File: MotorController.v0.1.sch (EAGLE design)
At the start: 47 parts, among them IC1 MC33035, IC2 MC33039

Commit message: Image + version.
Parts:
- removed R3B: 1M, resistor:R-EU_0204/2V
- added C2: 0.01uF, rcl:C-EU025-025X050
- added C6: 47uF, rcl:C-EU025-025X050
- added D5: 1N4148, diode:1N4148DO35-7
- added JP2: (no value), jumper:JP1E
- added LED1: (no value), led:LEDLD260
- added R10, R11: 2.2k, resistor:R-EU_0204/2V
- added R19: 4.7k, resistor:R-EU_0204/2V
- added SL2: (no value), con-amp-quick:M02
- R2: value 1M -> 5.1k
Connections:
- removed net FAULT: IC1.14
- new net FAULT_N: D5.C, IC1.14, LED1.C
- new net FOUT_: JP2.1, R3.1, TP1.TP
- new net FWD/REV: IC1.3, S1.S
- new net N$1: R19.1, S2.S
- new net N$11: C6.1, INC.3, R10.1, S4.S
- new net N$2: LED1.A, R11.1
- new net N$6: D5.A, R10.2
- new net OE: IC1.7, R19.2, S4.P
- new net OSC: C2.1, IC1.10, R2.1
- new net REFO: C6.2, IC1.8, INC.1, R2.2
- net FOUT: now also JP2.2; no longer R3.1
- net GND: now also C2.2, S1.P, S2.P, SL2.2
- net N$7: now also TP2.TP
- net VCC: now also R11.2, SL2.1
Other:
- moved on the sheet: C1, C3, C4, C5, C7, C8, D1, D2, D3, D4, IC1, IC2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

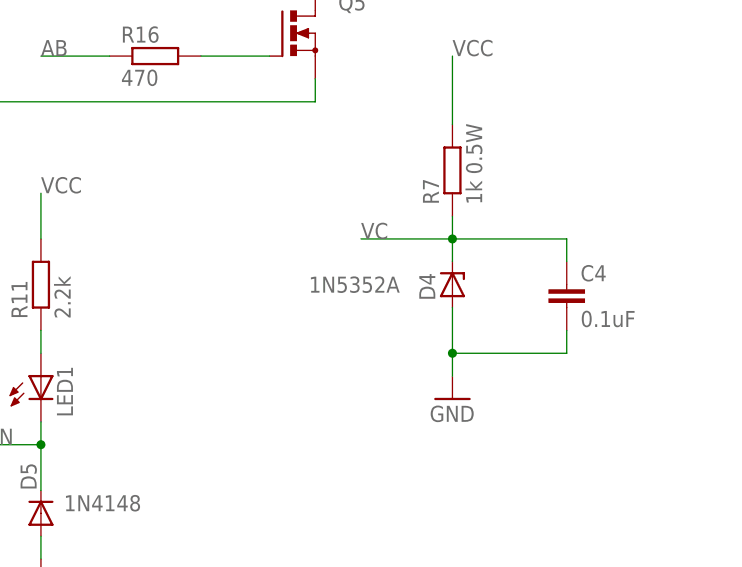
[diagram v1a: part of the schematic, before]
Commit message: Added board.
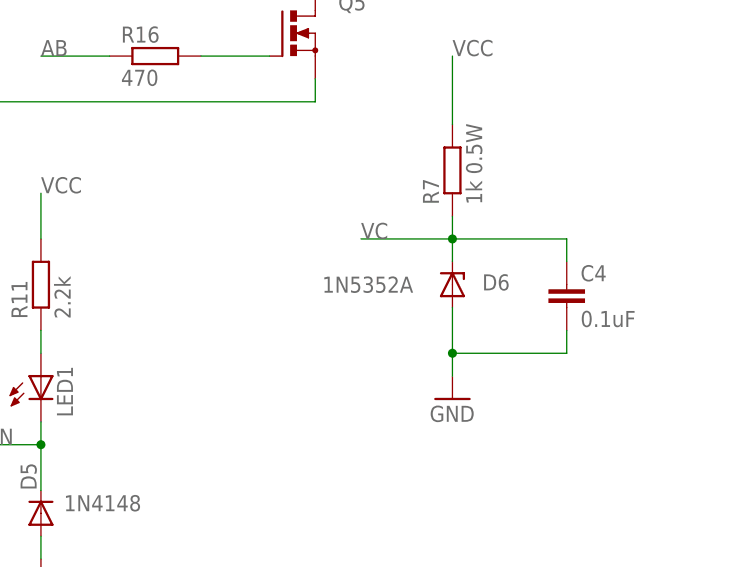
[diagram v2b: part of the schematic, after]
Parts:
- removed D4: 1N5352A, diode:1N5333
- added D6: 1N5352A, diode:BZV10
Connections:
- net GND: now also D6.A; no longer D4.A
- net VC: now also D6.C; no longer D4.C
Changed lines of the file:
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@@
 <part name="D3" library="diode" deviceset="1N4148" device="DO35-7" value="1N5819"/>
 <part name="GND4" library="supply1" deviceset="GND" device=""/>
-<part name="D4" library="diode" deviceset="1N5333" device="" value="1N5352A"/>
 <part name="C4" library="rcl" deviceset="C-EU" device="025-025X050" value="0.1uF"/>
 <part name="R7" library="resistor" deviceset="R-EU_" device="0204/2V" value="1k 0.5W"/>
@@
 <part name="JP2" library="jumper" deviceset="JP1E" device=""/>
 <part name="SL2" library="con-amp-quick" deviceset="M02" device=""/>
+<part name="D6" library="diode" deviceset="BZV10" device="" value="1N5352A"/>
 </parts>
 <sheets>
@@
 </instance>
 <instance part="GND4" gate="1" x="419.1" y="96.52"/>
-<instance part="D4" gate="1" x="518.16" y="157.48" smashed="yes" rot="R90">
-<attribute name="NAME" x="516.255" y="155.702" size="1.778" layer="95" rot="R90"/>
-<attribute name="VALUE" x="512.318" y="158.369" size="1.778" layer="96" rot="R180"/>
-</instance>
 <instance part="C4" gate="G$1" x="530.86" y="157.48"/>
 <instance part="R7" gate="G$1" x="518.16" y="170.18" rot="R90"/>
@@
 <instance part="JP2" gate="A" x="358.14" y="165.1" rot="R270"/>
 <instance part="SL2" gate="G$1" x="347.98" y="231.14" rot="R180"/>
+<instance part="D6" gate="1" x="518.16" y="157.48" smashed="yes" rot="R90">
+<attribute name="NAME" x="521.462" y="156.845" size="1.778" layer="95"/>
+<attribute name="VALUE" x="503.682" y="156.591" size="1.778" layer="96"/>
+</instance>
 </instances>
 <busses>
@@
 </segment>
 <segment>
-<pinref part="D4" gate="1" pin="A"/>
 <wire x1="518.16" y1="154.94" x2="518.16" y2="149.86" width="0.1524" layer="91"/>
 <wire x1="518.16" y1="149.86" x2="530.86" y2="149.86" width="0.1524" layer="91"/>
@@
 <wire x1="518.16" y1="147.32" x2="518.16" y2="149.86" width="0.1524" layer="91"/>
 <junction x="518.16" y="149.86"/>
+<pinref part="D6" gate="1" pin="A"/>
 </segment>
 <segment>
@@
 <segment>
 <pinref part="R7" gate="G$1" pin="1"/>
-<pinref part="D4" gate="1" pin="C"/>
 <wire x1="518.16" y1="165.1" x2="518.16" y2="162.56" width="0.1524" layer="91"/>
 <pinref part="C4" gate="G$1" pin="1"/>
@@
 <wire x1="518.16" y1="162.56" x2="508" y2="162.56" width="0.1524" layer="91"/>
 <label x="508" y="162.56" size="1.778" layer="95"/>
-</segment>
-</net>
+<pinref part="D6" gate="1" pin="C"/>
+</segment>
+</net>
